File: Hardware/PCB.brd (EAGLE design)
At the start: 170.2 x 111.2 mm, 103 parts, among them IC1 BD5229G-TR, IC4 XC6220A331MR-G, J1 FH34SRJ-24S-0.5SH_99_, J3 QWIIC_RIGHT_ANGLE, J4 112A-TAAR-R03_ATTEND, Q1 20V/4.2A/52mΩ/1.4W, Q2 20V/4.2A/52mΩ/1.4W, Q3 SI1308EDL-T1-GE3, U1 W25Q512JVEIQ, U2 ESP32-C6-WROOM-1-N8, U3 DS3231SN#, U4 MAX17048G+T10

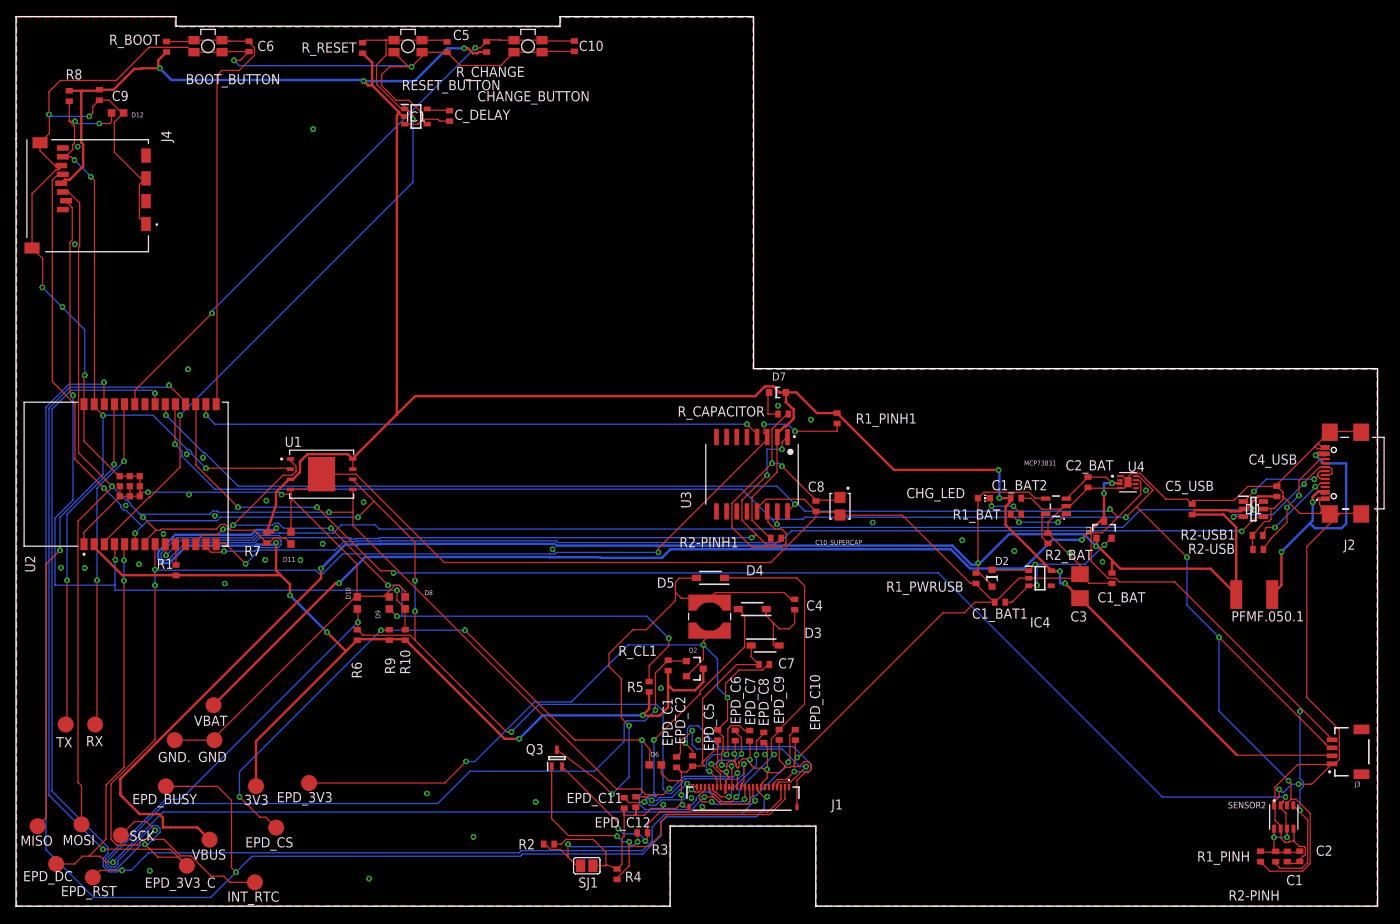
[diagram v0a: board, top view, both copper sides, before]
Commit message: add files
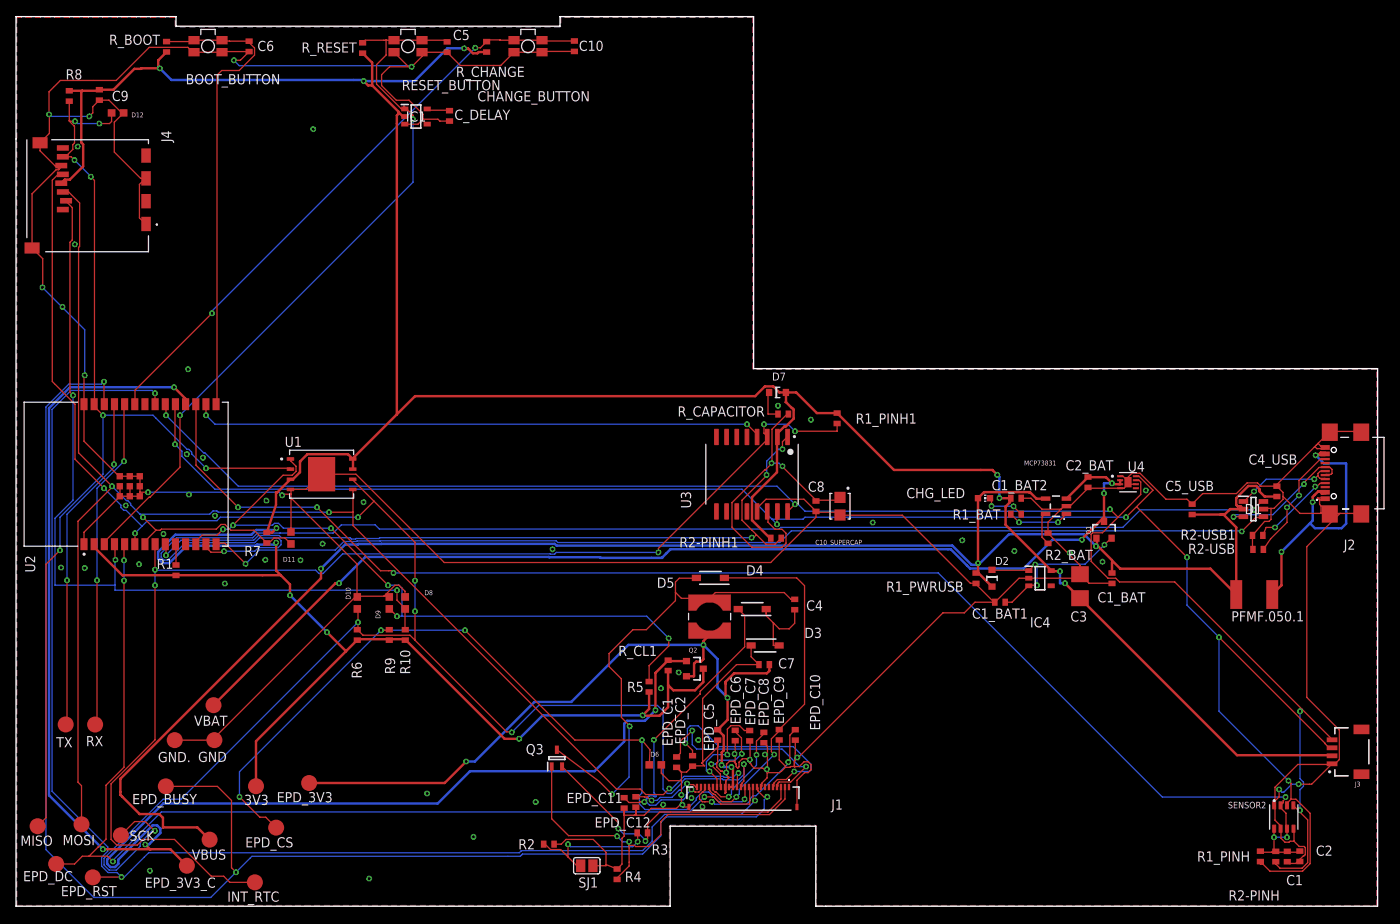
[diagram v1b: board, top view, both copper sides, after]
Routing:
- net EPD_3V3_C: track 194.5 -> 191.0 mm
- net EPD_3V3: track 92.9 -> 94.4 mm
- net 32KHZ: track 97.0 -> 96.2 mm
- net SCK: track 238.0 -> 238.6 mm
- net GND: track 725.7 -> 726.0 mm, vias 57 -> 58
